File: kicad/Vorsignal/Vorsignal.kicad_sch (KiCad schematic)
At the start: 7 parts, among them J0 VCC, J1 VkzBw, J3 GELB, J4 GRÜN

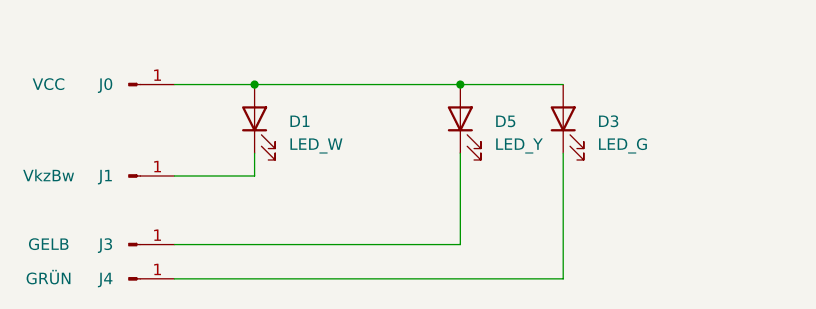
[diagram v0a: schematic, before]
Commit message: Add CC-BY-SA 4.0 license
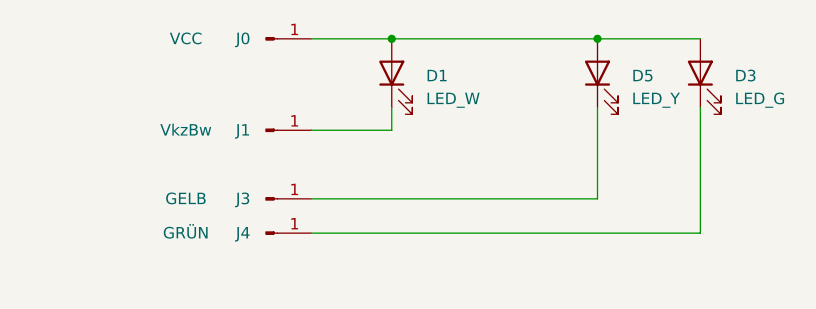
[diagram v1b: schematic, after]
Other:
- title: (none) -> KS-Vorsignal
- moved on the sheet: D1, D3, D5, J0, J1, J3, J4
